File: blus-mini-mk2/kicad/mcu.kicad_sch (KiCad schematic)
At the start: 21 parts, among them J1 USB_B, J12 REDFIT_SWD_10, SW1 BOOT, SW2 NRST, U6 STM32H723VGTx, U8 USBLC6-2SC6, U9 STM32F401RBTx

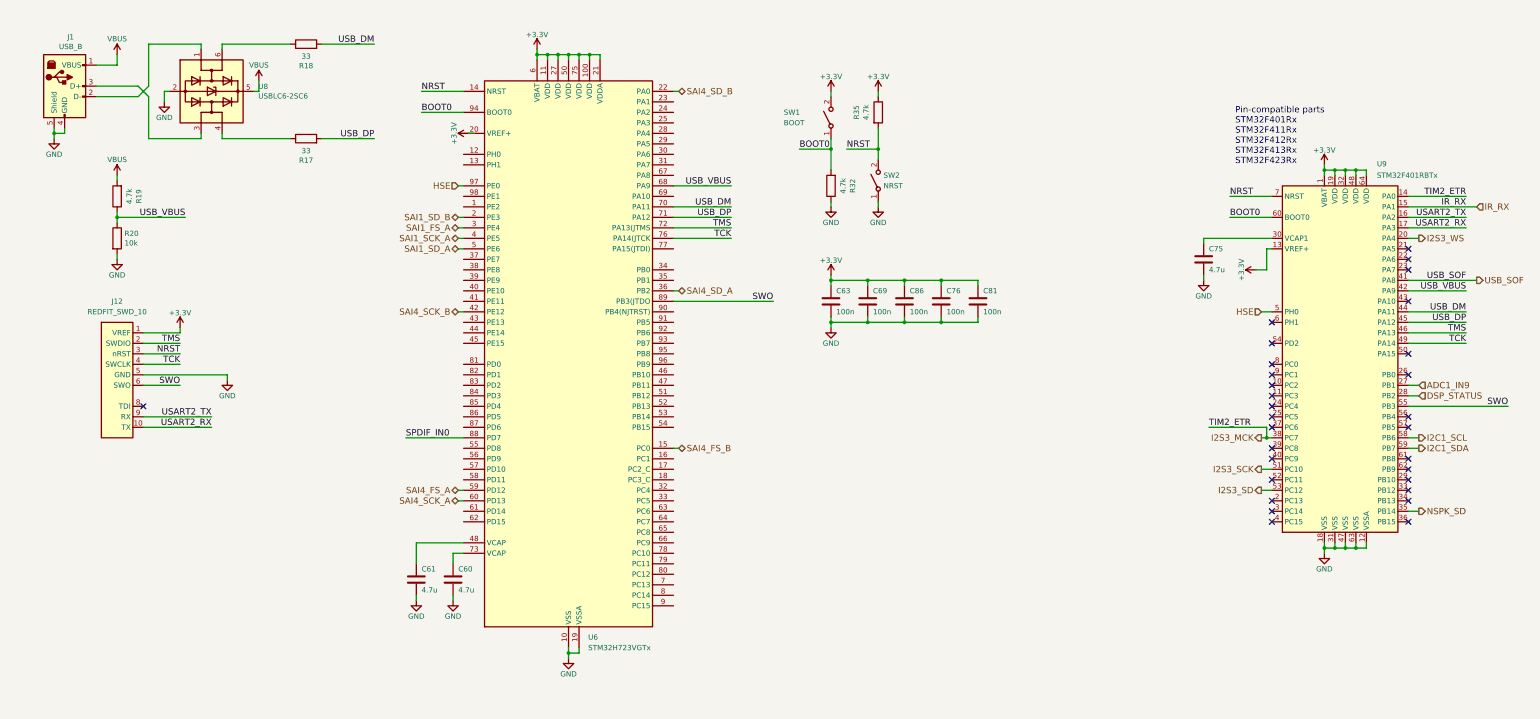
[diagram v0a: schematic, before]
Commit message: feat: wip, added most components
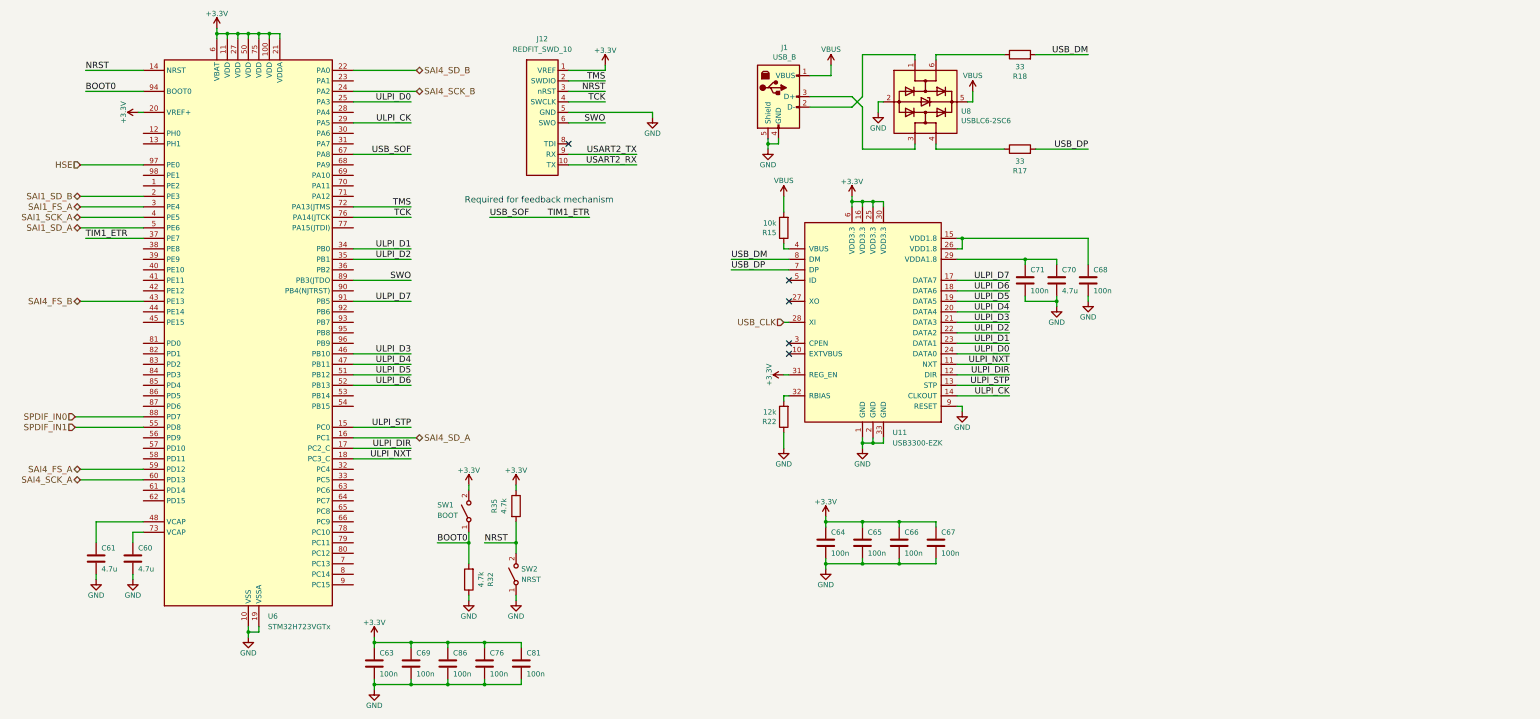
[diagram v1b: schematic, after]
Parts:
- removed C75: 4.7u, Capacitor_SMD:C_0805_2012Metric, symbol Device:C
- removed R19: 4.7k, Resistor_SMD:R_0402_1005Metric, symbol Device:R
- removed R20: 10k, Resistor_SMD:R_0402_1005Metric, symbol Device:R
- removed U9: STM32F401RBTx, Package_QFP:LQFP-64_10x10mm_P0.5mm, symbol MCU_ST_STM32F4:STM32F401RBTx
- added C64, C65, C66, C67, C68, C71: 100n, Capacitor_SMD:C_0402_1005Metric, symbol Device:C
- added C70: 4.7u, Capacitor_SMD:C_0805_2012Metric, symbol Device:C
- added R15: 10k, Resistor_SMD:R_0402_1005Metric, symbol Device:R
- added R22: 12k, Resistor_SMD:R_0402_1005Metric, symbol Device:R
- added U11: USB3300-EZK, Package_DFN_QFN:QFN-32-1EP_5x5mm_P0.5mm_EP3.45x3.45mm, symbol Interface_USB:USB3300-EZK
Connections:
- net +3.3V: now also U6.20 (VREF+), C64.1, C65.1, C66.1, C67.1, U11.16 (VDD3.3), U11.25 (VDD3.3), U11.30 (VDD3.3), U11.31 (REG_EN), U11.6 (VDD3.3)
- net GND: now also C64.2, C65.2, C66.2, C67.2, C68.2, C70.2, C71.2, R22.1, U11.1 (GND), U11.2 (GND), U11.33 (GND), U11.9 (RESET)
- net SAI4_FS_B: now also U6.43 (PE13); no longer U6.15 (PC0)
- net SAI4_SCK_B: now also U6.24 (PA2); no longer U6.42 (PE12)
- net SAI4_SD_A: now also U6.16 (PC1); no longer U6.36 (PB2)
- net USB_DM: now also U11.8 (DM); no longer U6.70 (PA11)
- net USB_DP: now also U11.7 (DP); no longer U6.71 (PA12)
- net VBUS: now also R15.2
- net ULPI_DIR: now reaches U6.17 (PC2_C)
- net ULPI_DIR: now also U11.12 (DIR)
- net ULPI_NXT: now reaches U6.18 (PC3_C)
- net ULPI_NXT: now also U11.11 (NXT)
- net ULPI_D0: now reaches U6.25 (PA3)
- net ULPI_D0: now also U11.24 (DATA0)
- net ULPI_CK: now reaches U6.29 (PA5)
- net ULPI_CK: now also U11.14 (CLKOUT)
- net ULPI_D1: now reaches U6.34 (PB0)
- net ULPI_D1: now also U11.23 (DATA1)
- net ULPI_D2: now reaches U6.35 (PB1)
- net ULPI_D2: now also U11.22 (DATA2)
- net TIM1_ETR: now reaches U6.37 (PE7)
- net TIM1_ETR: now also U6.67 (PA8)
- net ULPI_D3: now reaches U6.46 (PB10)
- net ULPI_D3: now also U11.21 (DATA3)
- net ULPI_D4: now reaches U6.47 (PB11)
- net ULPI_D4: now also U11.20 (DATA4)
- net ULPI_D5: now reaches U6.51 (PB12)
- net ULPI_D5: now also U11.19 (DATA5)
- net ULPI_D6: now reaches U6.52 (PB13)
- net ULPI_D6: now also U11.18 (DATA6)
- net SPDIF_IN1: now reaches U6.55 (PD8)
- net ULPI_D7: now reaches U6.91 (PB5)
- net ULPI_D7: now also U11.17 (DATA7)
- net USB_VBUS: no longer names the net of U6.68 (PA9)
- new net: R22.2, U11.32 (RBIAS)
- new net: C68.1, U11.15 (VDD1.8), U11.26 (VDD1.8)
- new net: C70.1, C71.1, U11.29 (VDDA1.8)
- new net: R15.1, U11.4 (VBUS)
- new net ULPI_STP: U11.13 (STP), U6.15 (PC0)
- new net USB_CLK: U11.28 (XI)
- no-connect marks 30 -> 5
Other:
- note added: "Required for feedback mechanism"
- note removed: "Pin-compatible parts STM32F401Rx STM32F411Rx STM32F412Rx STM32F413Rx STM32F423Rx"
- moved on the sheet: C60, C61, C63, C69, C76, C81, C86, J1, J12, R17, R18, R32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
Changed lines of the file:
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@@
-(kicad_sch (version 20230121) (generator eeschema)
-  (paper "A4")
-  (title_block
-    (title "blus mini mk2")
-    (date "2024-04-05")
-    (rev "a")
-    (company "elagil")
-  )
+(kicad_sch
+	(version 20231120)
+	(generator "eeschema")
+	(generator_version "8.0")
+	(paper "A4")
+	(title_block
+		(title "blus mini mk2")
+		(date "2024-04-05")
+		(rev "a")
+		(company "elagil")
+	)
